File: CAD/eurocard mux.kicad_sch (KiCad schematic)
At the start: 3 parts, among them J1 Conn_01x16, J2 Conn_01x16, J3 1847712

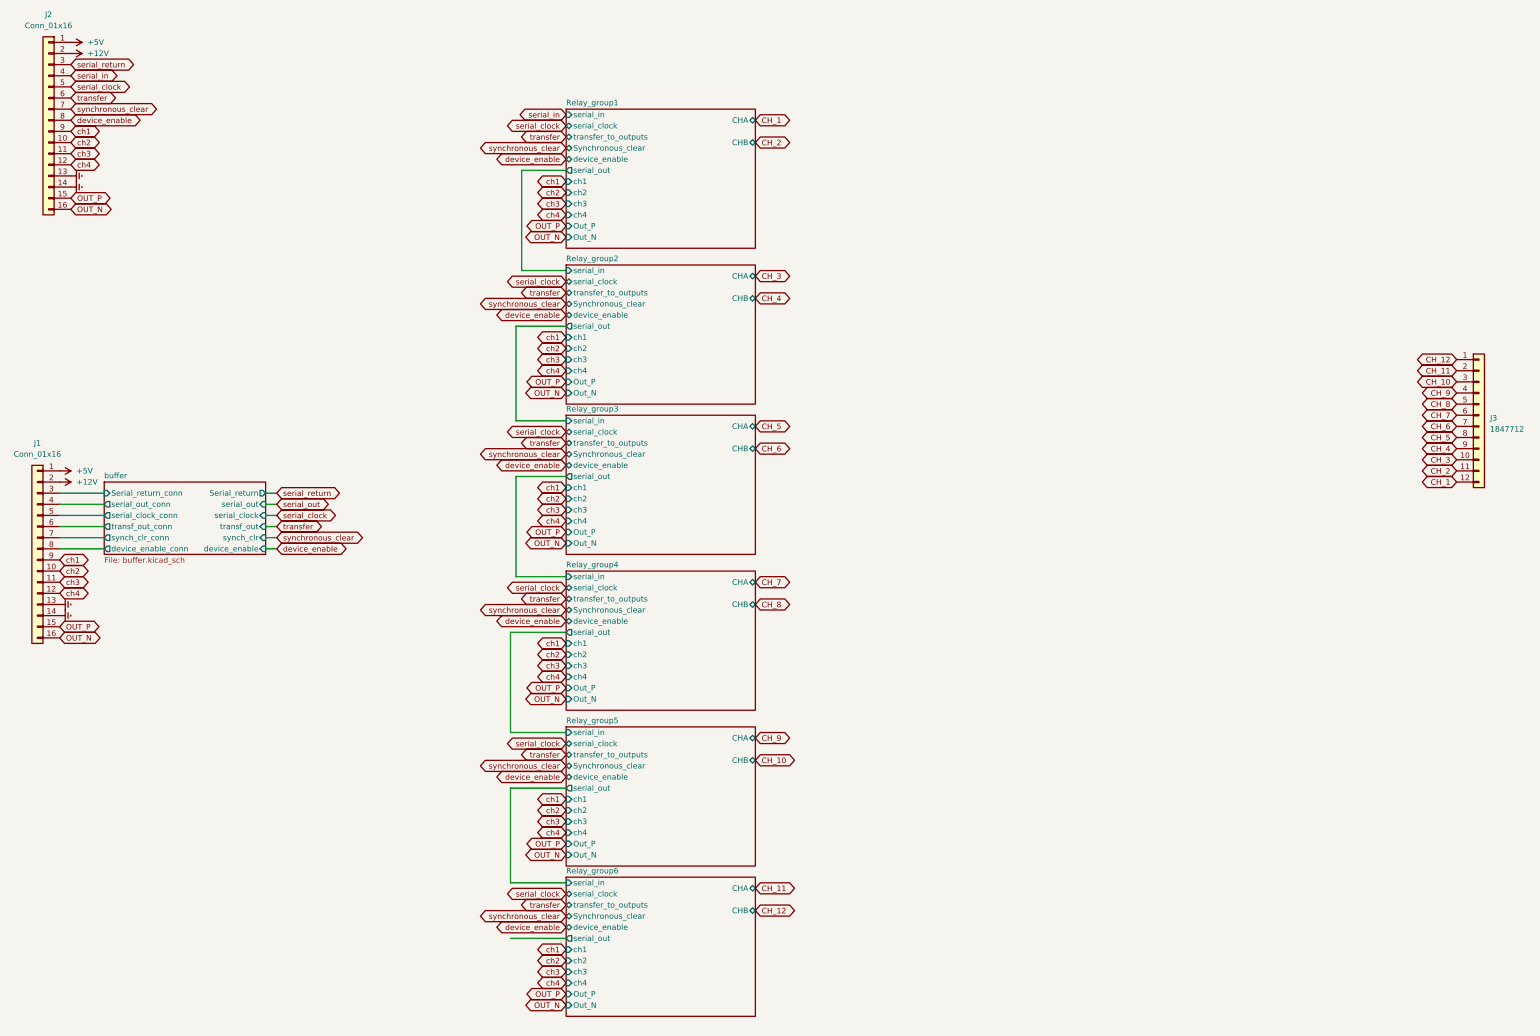
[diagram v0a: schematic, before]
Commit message: Feat: WIP
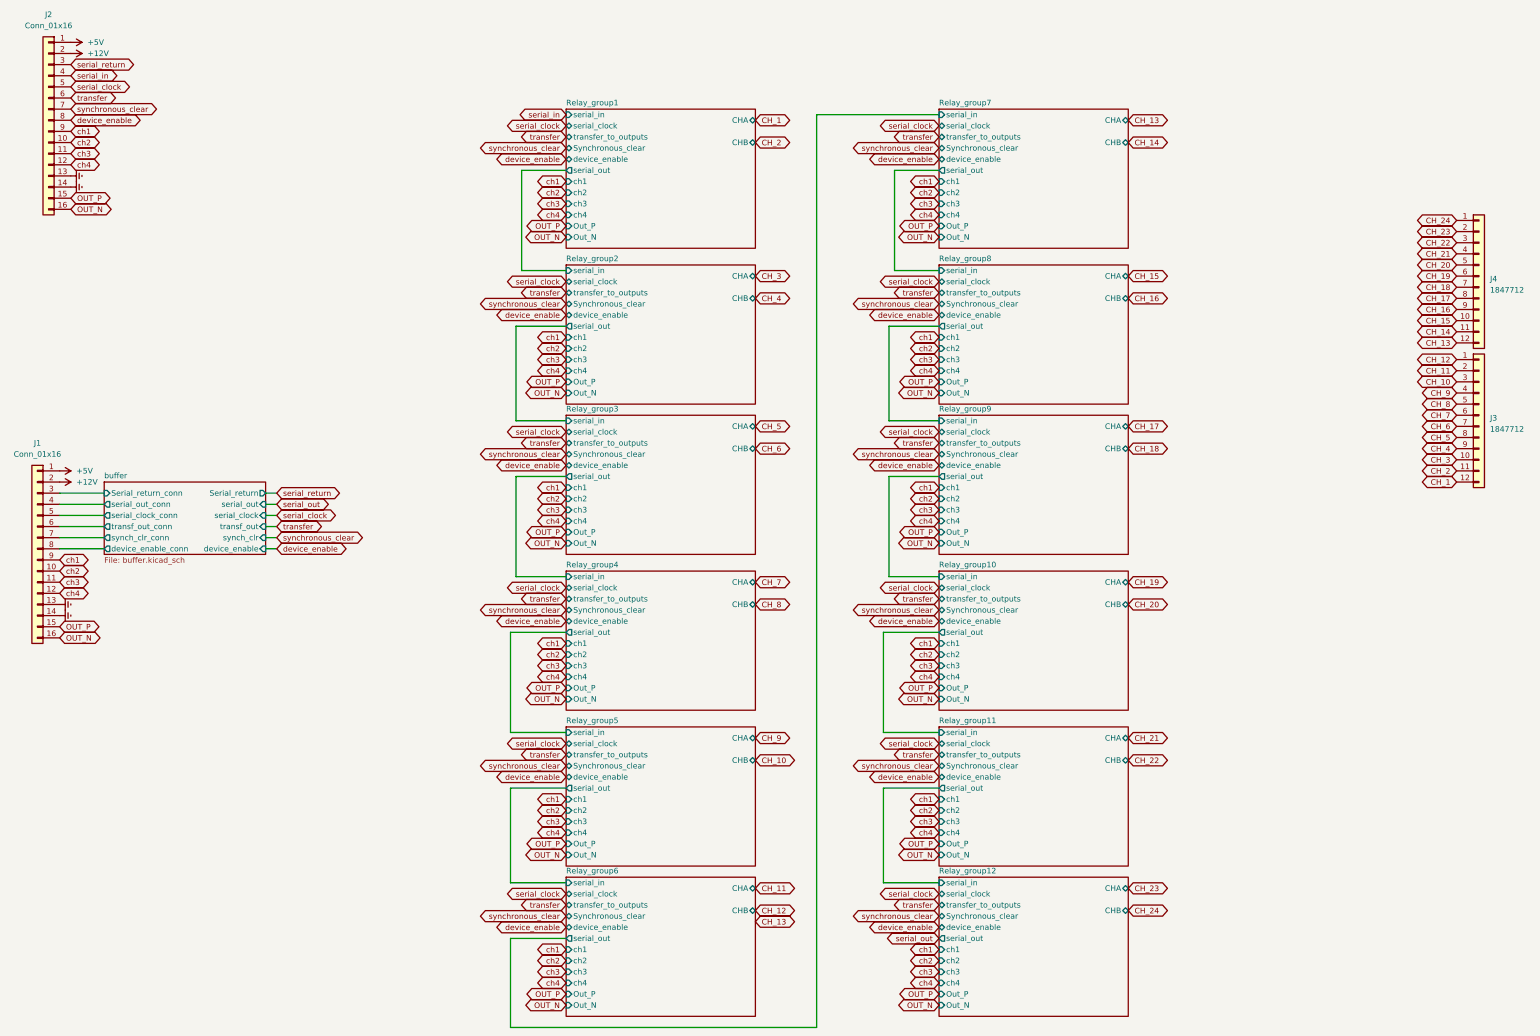
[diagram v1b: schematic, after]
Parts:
- added J4: 1847712, Connector_Phoenix_MC_HighVoltage:PhoenixContact_MC_1,5_12-GF-5.08_1x12_P5.08mm_Horizontal_ThreadedFlange_MountHole, symbol Connector_Generic:Conn_01x12
- J1, J2: footprint Connector_IDC:IDC-Header_2x08_P2.54mm_Vertical -> Connector_IDC:IDC-Header_2x08_P2.54mm_Horizontal
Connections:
- new net CH_13: J4.12 (Pin_12)
- new net CH_14: J4.11 (Pin_11)
- new net CH_15: J4.10 (Pin_10)
- new net CH_16: J4.9 (Pin_9)
- new net CH_17: J4.8 (Pin_8)
- new net CH_18: J4.7 (Pin_7)
- new net CH_19: J4.6 (Pin_6)
- new net CH_20: J4.5 (Pin_5)
- new net CH_21: J4.4 (Pin_4)
- new net CH_22: J4.3 (Pin_3)
- new net CH_23: J4.2 (Pin_2)
- new net CH_24: J4.1 (Pin_1)
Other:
- added sheet Relay_group10 (Relay_group.kicad_sch)
- added sheet Relay_group11 (Relay_group.kicad_sch)
- added sheet Relay_group12 (Relay_group.kicad_sch)
- added sheet Relay_group7 (Relay_group.kicad_sch)
- added sheet Relay_group8 (Relay_group.kicad_sch)
- added sheet Relay_group9 (Relay_group.kicad_sch)
